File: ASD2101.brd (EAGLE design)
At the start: 22.5 x 22.5 mm, 16 parts, among them J1 20021111, J2 DF12-32-DS, J3 47346-0001, J4 DF12-32-DP, Q1 DMP2035U, U1 FT232RQ

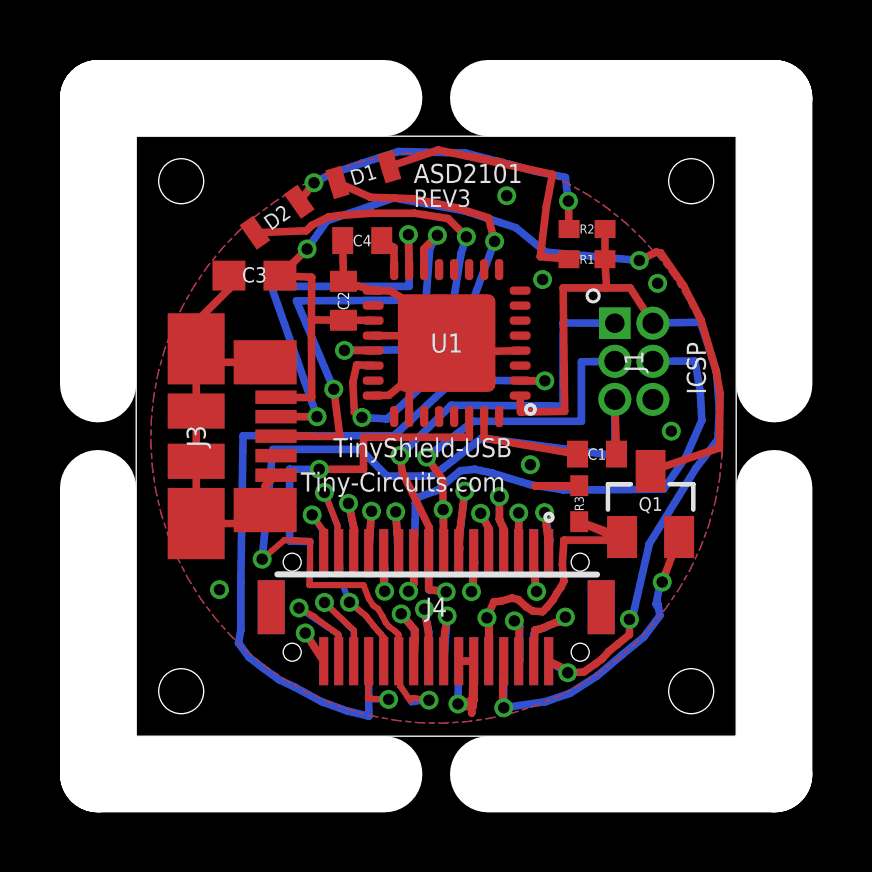
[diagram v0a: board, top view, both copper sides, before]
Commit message: Updated to Rev4
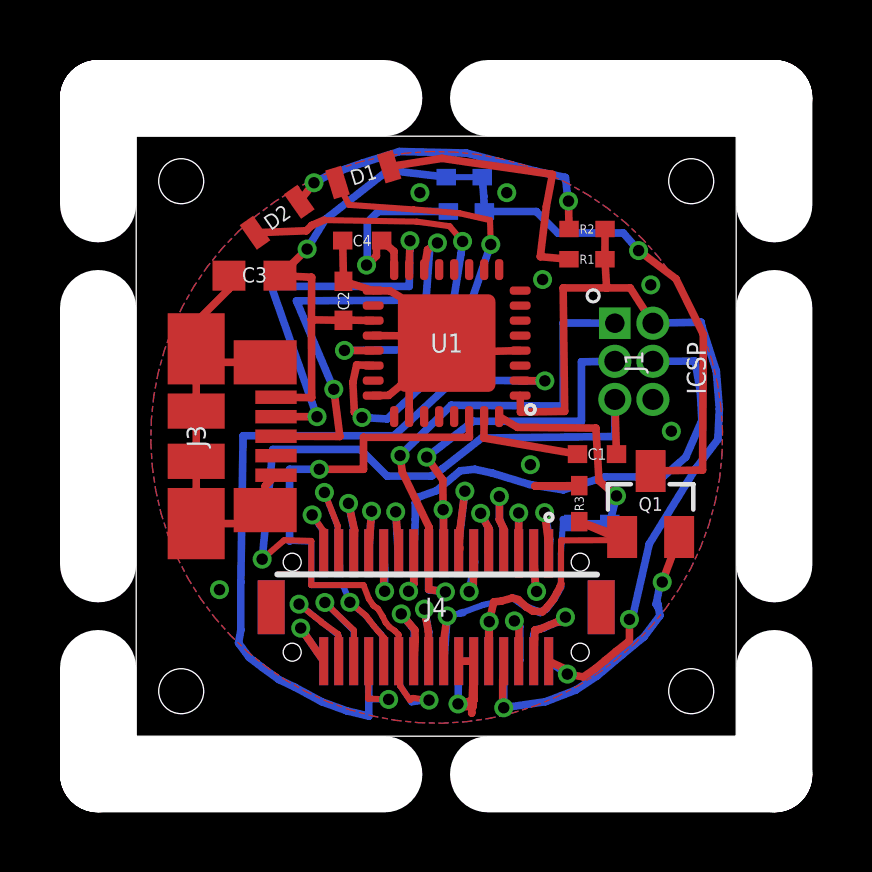
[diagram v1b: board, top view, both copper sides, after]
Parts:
- added R4, R6: 0.0, tinycircuits:0402_SHORT
- added R5: 0.0, tinycircuits:0402
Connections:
- removed net N$1: C4.1, U1.16
- new net 3V3OUT: C4.1, R5.1, U1.16
- new net N$4: Q1.3, R4.2, R5.2
- new net RTS: R6.1, U1.32
- net RSV2: now also R6.2
- net USBVCC: now also R4.1; no longer Q1.3
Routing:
- net N$4: track 0.00 -> 16.7 mm, vias 0 -> 1
- net USBVCC: track 31.9 -> 15.4 mm, vias 2 -> 1
- net RSV2: track 3.04 -> 10.2 mm
- net RTS: track 0.00 -> 6.78 mm, vias 0 -> 1
- net 3V3OUT: track 0.00 -> 6.48 mm, vias 0 -> 1
- net N$1: track 1.21 -> 0.00 mm
- net RESET: track 31.8 -> 31.1 mm
- net GND: vias 7 -> 8
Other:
- outline, holes or cut-outs redrawn
- board text added: "4"
- board text added: "ASD2101 - Rev4"
- board text added: "R4"
- board text added: "R5"
- board text added: "R6"
- board text added: "USB TinyShield"
- board text removed: "3"
- board text removed: "ASD2101"
- board text removed: "REV3"
- board text removed: "TinyShield-USB"

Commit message: Updated to Rev 6
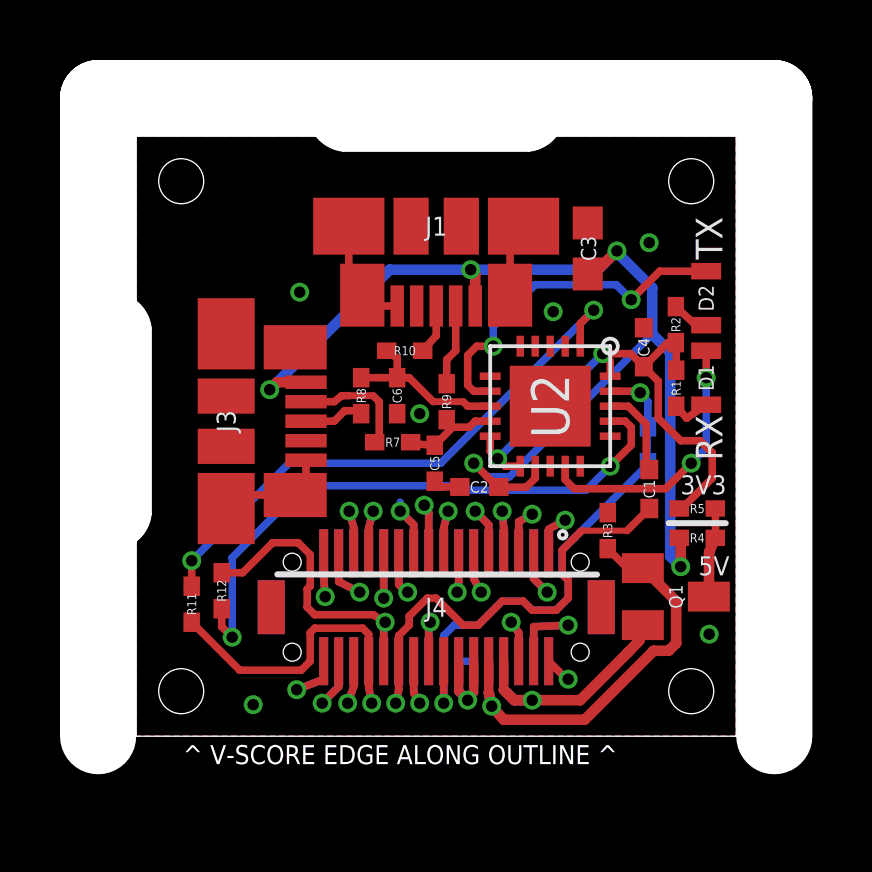
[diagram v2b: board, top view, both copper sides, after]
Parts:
- removed U1: FT232RQ, tinycircuits:MLF32
- added C5, C6: 47pF, tinycircuits:0402
- added R10, R7, R8, R9: 27.0, tinycircuits:0402
- added R11, R12: 1.00K, tinycircuits:0402
- added U2: FT231XQ-R, tinycircuits:QFN20
- J1: value 20021111 -> 47346-0001; device tinycircuits:2X3_.05"_TH_HEADER -> tinycircuits:MICRO_USB
- R4: device tinycircuits:0402_SHORT -> tinycircuits:0402
- moved D2 14.6 mm to (29.0, 24.6), turned to 180 degrees
- moved R4 14.3 mm to (28.7, 16.6), flipped to the top, turned to 0 degrees
- moved D1 13.3 mm to (29.0, 21.9), turned to 180 degrees
- moved R5 12.5 mm to (28.7, 17.6), flipped to the top, turned to 0 degrees
- moved C3 11.1 mm to (25.1, 26.3), turned to 90 degrees
- moved C4 10.0 mm to (26.9, 23.0), turned to 90 degrees
- moved J1 7.98 mm to (20.0, 27.0), turned to 270 degrees
- moved C2 7.68 mm to (21.4, 18.3), turned to 180 degrees
- moved R1 5.23 mm to (28.0, 21.6), turned to 90 degrees
- moved R2 4.35 mm to (28.0, 23.7), turned to 270 degrees
- moved R6 3.21 mm to (27.1, 19.7), turned to 270 degrees
- moved Q1 3.20 mm to (28.0, 14.7), turned to 270 degrees
- moved C1 2.10 mm to (27.1, 18.2), turned to 270 degrees
- moved R3 1.31 mm to (25.7, 16.9)
- moved J3 1.12 mm to (13.0, 20.5)
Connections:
- removed net N$13: J3.3, U1.14
- new net N$1: J3.2, R7.1
- new net N$10: R12.2, U2.17
- new net N$3: J1.3, R10.1
- new net N$8: J3.3, R8.1
- new net N$9: R11.2, U2.1
- new net USBDM: C5.1, R7.2, R9.2, U2.9
- new net USBDP: C6.1, R10.2, R8.2, U2.8
- net +5V: now also Q1.E; no longer Q1.2
- net 3V3OUT: now also R1.2, R2.2, U2.10, U2.11, U2.20; no longer U1.16
- net DTR: now also U2.18; no longer U1.31
- net GND: now also C5.2, C6.2, J1.5, J1.P1, J1.P2, J1.P3, J1.P4, J1.P5, J1.P6, U2.13, U2.21, U2.3; no longer J1.6, U1.17, U1.20, U1.24, U1.26, U1.33, U1.4
- net IO0: now also R12.1; no longer U1.30
- net IO1: now also R11.1; no longer U1.2
- net MISO: no longer J1.1
- net MOSI: no longer J1.4
- net N$16: now also U2.14; no longer U1.22
- net N$2: now also J1.2, R9.1; no longer J3.2, U1.15
- net N$4: now also Q1.C; no longer Q1.3
- net N$5: now also U2.7; no longer U1.21
- net RESET: no longer J1.5
- net RTS: now also U2.19; no longer U1.32
- net SCK: no longer J1.3
- net USBVCC: now also J1.1, U2.12; no longer U1.19
- net VCC: no longer J1.2, R1.2, R2.2, U1.1
- net VIN: now also Q1.B; no longer Q1.1
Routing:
- net VCC: track 28.9 -> 1.80 mm, vias 2 -> 1
- net USBVCC: track 15.4 -> 40.9 mm, vias 1 -> 5
- net GND: track 41.4 -> 16.5 mm, vias 8 -> 7
- net N$10: track 0.00 -> 20.1 mm, vias 0 -> 2
- net N$9: track 0.00 -> 19.1 mm, vias 0 -> 2
- net IO1: track 29.5 -> 11.5 mm, vias 2 -> 1
- net MOSI: track 18.9 -> 3.47 mm
- net RESET: track 31.1 -> 16.2 mm, vias 2 -> 1
- net N$13: track 14.3 -> 0.00 mm, vias 2 -> 0
- net MISO: track 17.6 -> 3.28 mm, vias 2 -> 1
- net N$4: track 16.7 -> 2.98 mm, vias 1 -> 0
- net 3V3OUT: track 6.48 -> 18.1 mm, vias 1 -> 2
- net SCK: track 13.5 -> 2.84 mm, vias 2 -> 1
- net N$2: track 13.1 -> 2.71 mm, vias 2 -> 0
- net N$7: track 11.2 -> 1.25 mm, vias 2 -> 0
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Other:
- board size 22.5 x 22.5 mm -> 22.5 x 21.3 mm
- board text added: "3V3"
- board text added: "5V"
- board text added: "6"
- board text added: "ASD2101 - Rev6"
- board text added: "RX"
- board text added: "TX"
- board text added: "^ V-SCORE EDGE ALONG OUTLINE ^"
- board text removed: "4"
- board text removed: "ASD2101 - Rev4"
- board text removed: "ICSP"
- board text removed: "R4"
- board text removed: "R5"
